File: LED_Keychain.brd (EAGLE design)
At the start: 160 x 100 mm, 2 parts

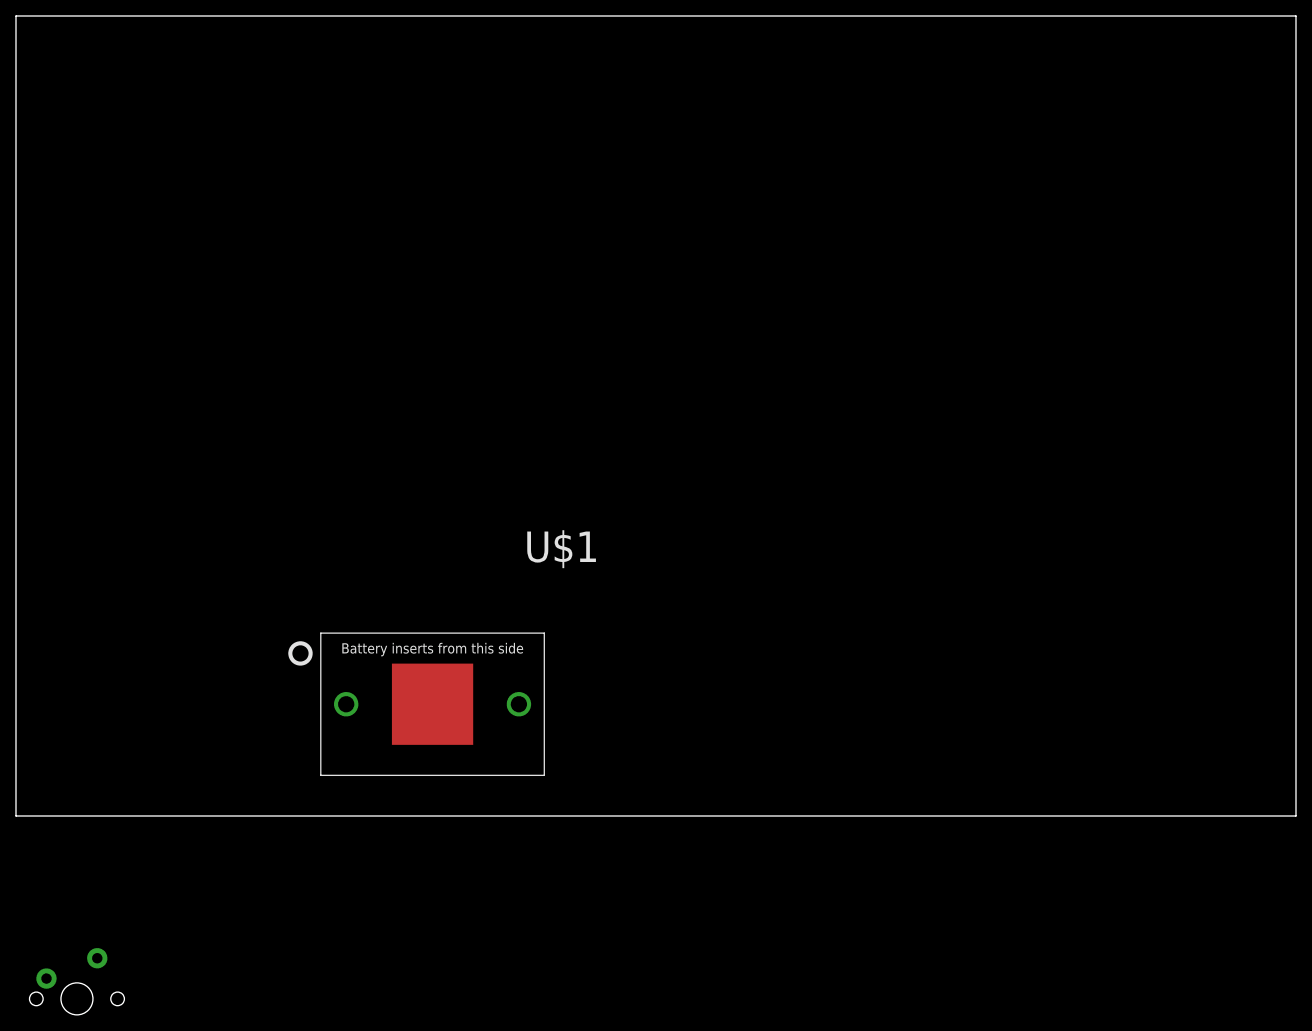
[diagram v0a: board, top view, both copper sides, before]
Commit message: Added Datasheet and made board changes
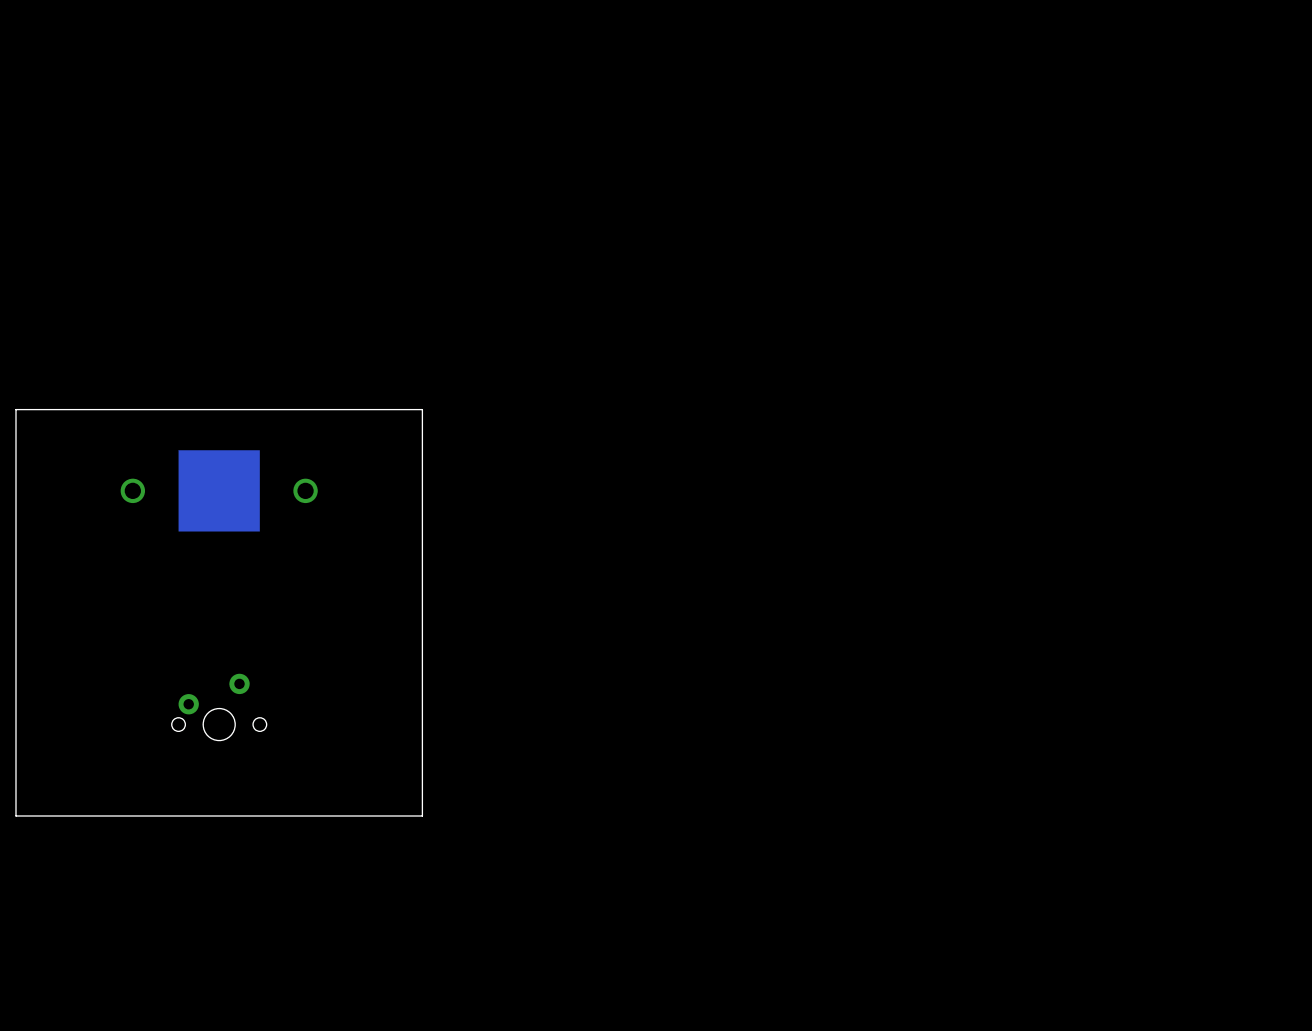
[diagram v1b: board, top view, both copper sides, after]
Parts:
- moved U$2 38.6 mm to (25.4, 11.4)
- moved U$1 37.7 mm to (25.4, 40.6), flipped to the bottom
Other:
- board size 160 x 100 mm -> 50.8 x 50.8 mm
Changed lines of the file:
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@@
 <board>
 <plain>
-<wire x1="0" y1="0" x2="160" y2="0" width="0" layer="20"/>
-<wire x1="160" y1="0" x2="160" y2="100" width="0" layer="20"/>
-<wire x1="160" y1="100" x2="0" y2="100" width="0" layer="20"/>
-<wire x1="0" y1="100" x2="0" y2="0" width="0" layer="20"/>
+<wire x1="0" y1="0" x2="50.8" y2="0" width="0" layer="20"/>
+<wire x1="50.8" y1="0" x2="50.8" y2="50.8" width="0" layer="20"/>
+<wire x1="50.8" y1="50.8" x2="0" y2="50.8" width="0" layer="20"/>
+<wire x1="0" y1="50.8" x2="0" y2="0" width="0" layer="20"/>
 </plain>
 <attributes>
@@
 </autorouter>
 <elements>
-<element name="U$2" library="Keyboard" package="MX-1U" value="KEYSWITCH-PLAIN-MX-1U" x="7.62" y="-22.86" smashed="yes">
-<attribute name="NAME" x="7.62" y="-25.66" size="1" layer="21" font="vector" ratio="13" align="center"/>
-<attribute name="NAME" x="7.62" y="-25.66" size="1" layer="22" font="vector" ratio="13" rot="MR0" align="center"/>
+<element name="U$2" library="Keyboard" package="MX-1U" value="KEYSWITCH-PLAIN-MX-1U" x="25.4" y="11.43" smashed="yes">
+<attribute name="NAME" x="25.4" y="8.63" size="1" layer="21" font="vector" ratio="13" align="center"/>
+<attribute name="NAME" x="25.4" y="8.63" size="1" layer="22" font="vector" ratio="13" rot="MR0" align="center"/>
 </element>
-<element name="U$1" library="LED_Keychain_lib" package="KEYSTONE3035" value="KEYSTONE3035" x="52.07" y="13.97" smashed="yes">
-<attribute name="NAME" x="63.5" y="31.75" size="3.81" layer="25"/>
+<element name="U$1" library="LED_Keychain_lib" package="KEYSTONE3035" value="KEYSTONE3035" x="25.4" y="40.64" smashed="yes" rot="MR0">
+<attribute name="NAME" x="13.97" y="58.42" size="3.81" layer="26" rot="MR0"/>
 </element>
 </elements>
